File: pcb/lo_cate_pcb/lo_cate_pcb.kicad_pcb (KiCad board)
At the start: 2 copper layers, 100 x 47.5 mm, 49 parts, among them J1 Conn_01x07_Pin, J2 690-005-299-043, J3 U.FL-R-SMT-110, SW1 MICRO_RESET, SW2 MICRO_ON, SW3 BUTTON1, SW4 BUTTON2, SW5 BUTTON3, U1 STM32F401RETx, U2 BMI323, U3 LED1, U4 LED2, U5 LED3, U6 RFM95W-868S2, U7 LDK320AM33R

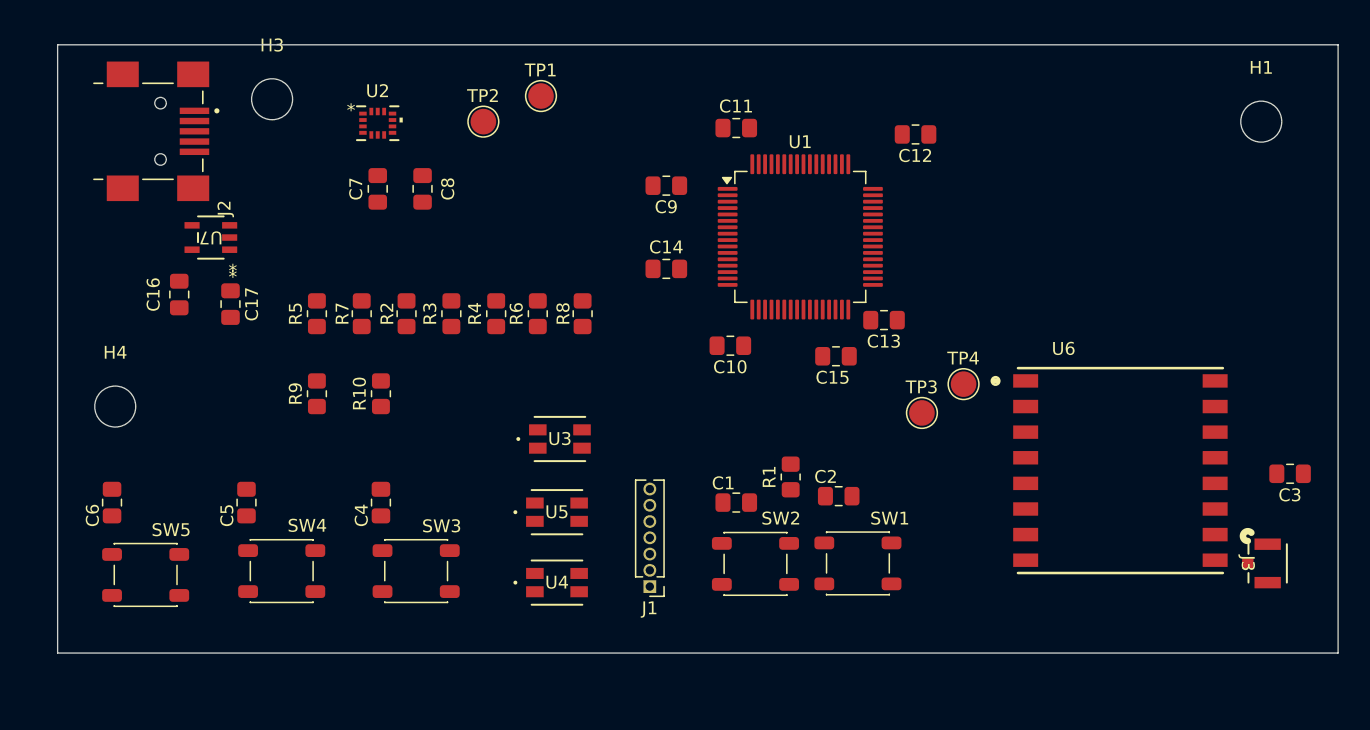
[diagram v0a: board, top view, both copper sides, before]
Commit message: Most PCB Routing is complete
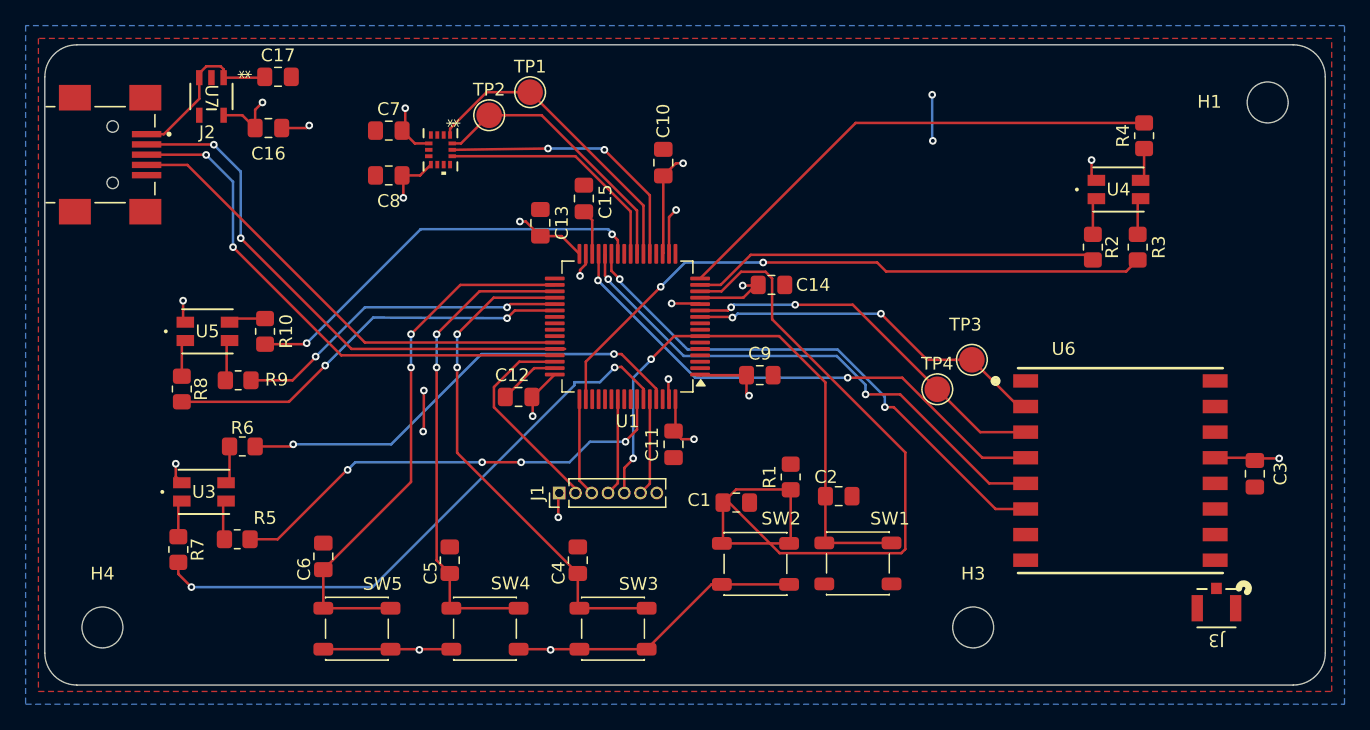
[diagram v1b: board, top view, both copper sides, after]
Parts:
- moved H3 68.6 mm to (230.0, 143.0)
- moved R2 53.9 mm to (239.3, 113.3), turned to 90 degrees
- moved R3 53.9 mm to (242.8, 113.3), turned to -90 degrees
- moved U4 53.5 mm to (241.3, 108.8)
- moved R4 52.5 mm to (243.3, 104.6)
- moved C12 37.2 mm to (194.5, 125.0), turned to 0 degrees
- moved R8 31.8 mm to (168.2, 124.4), turned to 90 degrees
- moved U5 30.7 mm to (170.2, 119.9)
- moved U3 28.1 mm to (169.9, 132.4)
- moved C13 27.9 mm to (196.2, 111.4), turned to -90 degrees
- moved R6 25.3 mm to (172.9, 128.9), turned to 0 degrees
- moved C11 25.2 mm to (206.6, 128.7), turned to 90 degrees
- moved R7 23.3 mm to (167.9, 136.9), turned to 90 degrees
- moved C15 23.2 mm to (199.6, 109.5), turned to 90 degrees
- moved R5 18.7 mm to (172.5, 136.1), turned to 0 degrees
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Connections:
- C16 pad 1: /3v3 -> /3V3
- U7 pad 5: /3v3 -> /3V3
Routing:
- net /3V3: track 0.00 -> 96.5 mm, vias 0 -> 18
- net /MICRO_WAKEUP: track 0.00 -> 66.5 mm
- net /LED2_RED: track 0.00 -> 50.0 mm, vias 0 -> 2
- net /LED1_BLUE: track 0.00 -> 46.5 mm, vias 0 -> 2
- net /NRST: track 0.00 -> 45.2 mm, vias 0 -> 2
- net /USB_DM: track 0.00 -> 43.0 mm, vias 0 -> 2
- net /BUTTON3: track 0.00 -> 42.3 mm, vias 0 -> 2
- net /LORA_RST: track 0.00 -> 42.1 mm, vias 0 -> 2
- net /LORA_CSB: track 0.00 -> 41.8 mm, vias 0 -> 2
- net /USB_DP: track 0.00 -> 41.5 mm, vias 0 -> 2
- net /LORA_SCK: track 0.00 -> 41.2 mm, vias 0 -> 2
- net /LED2_GREEN: track 0.00 -> 39.7 mm
- net /BUTTON1: track 0.00 -> 39.4 mm, vias 0 -> 2
- net /BUTTON2: track 0.00 -> 37.8 mm, vias 0 -> 2
- net /USB_ID: track 0.00 -> 37.8 mm
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- added copper zone on B.Cu, net /3V3
- added copper zone on F.Cu, net GND
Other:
- board size 100 x 47.5 mm -> 100 x 50 mm
